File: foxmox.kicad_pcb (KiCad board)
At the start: 2 copper layers, 63.5 x 63.5 mm, 17 parts, among them P1 2.5mm plug, Q1 2N2222A, U1 PIC16F84, Y1 3.579MHz

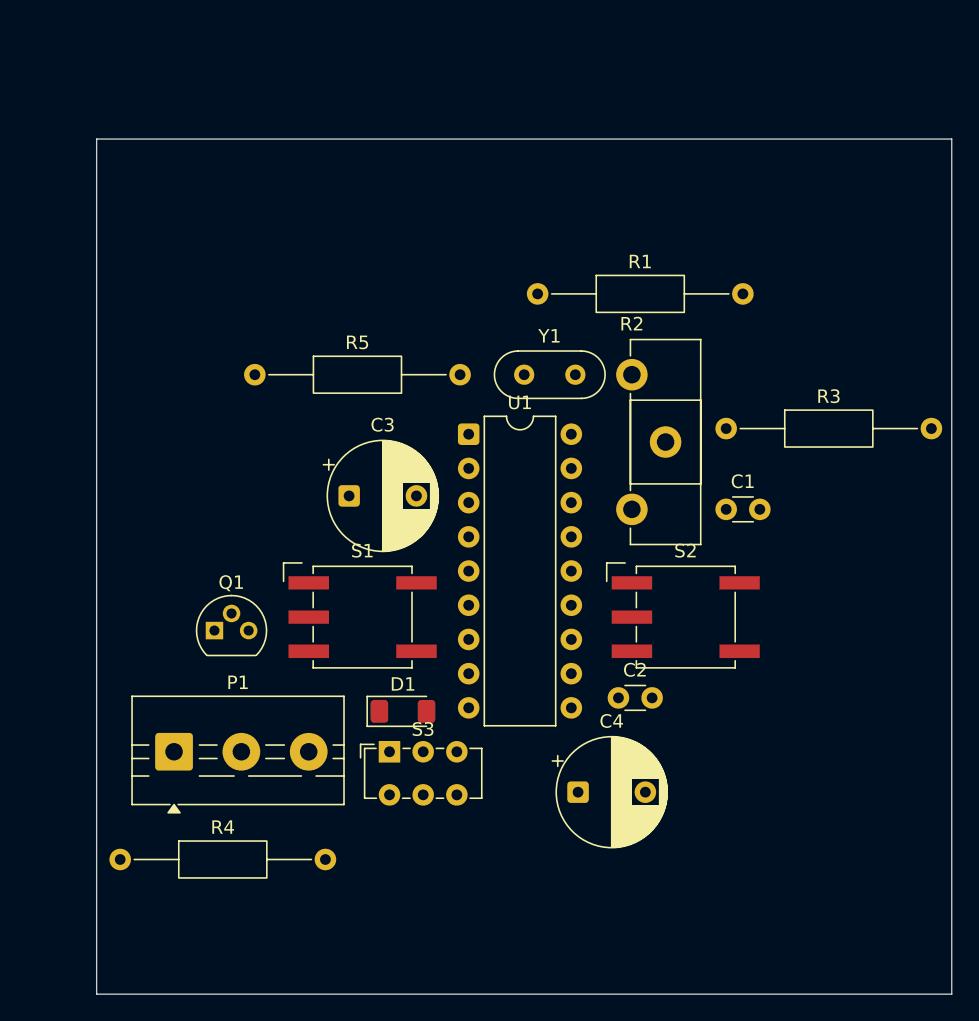
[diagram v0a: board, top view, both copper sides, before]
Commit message: Slightly better PCB
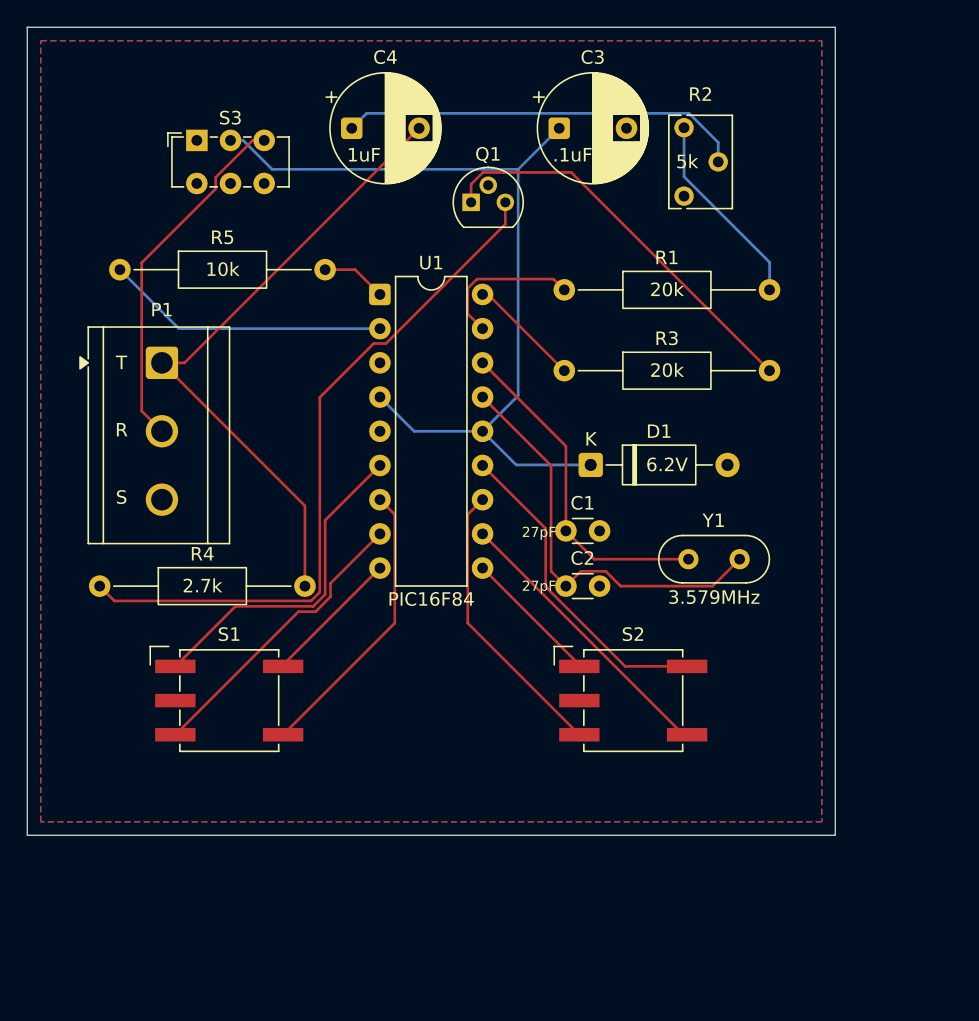
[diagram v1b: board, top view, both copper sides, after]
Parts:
- D1: footprint Diode_SMD:D_MiniMELF -> Diode_THT:D_A-405_P10.16mm_Horizontal
- P1: footprint TerminalBlock:TerminalBlock_MaiXu_MX126-5.0-03P_1x03_P5.00mm -> TerminalBlock_CUI:TerminalBlock_CUI_TB007-508-03_1x03_P5.08mm_Horizontal
- R2: footprint Potentiometer_THT:Potentiometer_Piher_PT-15-H01_Horizontal -> Potentiometer_THT:Potentiometer_Bourns_3266W_Vertical
- moved C4 52.1 mm to (134.1, 67.5)
- moved S3 47.6 mm to (122.6, 68.4)
- moved Q1 37.1 mm to (143.0, 73.0)
- moved C3 31.4 mm to (149.5, 67.5)
- moved P1 28.9 mm to (120.0, 84.9), turned to -90 degrees
- moved D1 23.0 mm to (151.8, 92.5)
- moved R4 20.4 mm to (115.4, 101.5)
- moved R2 18.7 mm to (158.8, 67.5), turned to 90 degrees
- moved Y1 18.3 mm to (159.1, 99.5)
- moved R3 12.8 mm to (149.9, 85.5)
- moved R5 12.7 mm to (116.9, 78.0)
- moved U1 12.3 mm to (136.2, 79.8)
- moved C1 12.0 mm to (150.0, 97.4)
- moved S1 11.7 mm to (125.0, 110.0)
- moved C2 9.17 mm to (150.0, 101.5)
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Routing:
- net Net-(D1-K): track 0.00 -> 64.8 mm, vias 0 -> 1
- net Net-(Q1-PadC): track 0.00 -> 52.3 mm
- net Net-(C4-Pad2): track 0.00 -> 47.3 mm
- net Net-(U1-OSC1/CLKIN): track 0.00 -> 31.2 mm
- net Net-(C4-Pad1): track 0.00 -> 30.0 mm
- net Net-(Q1-PadB): track 0.00 -> 30.0 mm
- net Net-(S3-C): track 0.00 -> 26.5 mm
- net Net-(U1-OSC2/CLKOUT): track 0.00 -> 25.0 mm
- net Net-(U1-INT/RB0): track 0.00 -> 24.6 mm
- net Net-(U1-RB7): track 0.00 -> 23.9 mm
- net Net-(U1-RB2): track 0.00 -> 22.0 mm
- net Net-(U1-RB5): track 0.00 -> 21.4 mm
- net Net-(U1-RB6): track 0.00 -> 21.3 mm
- net Net-(U1-RB1): track 0.00 -> 21.3 mm
- net Net-(U1-RA3): track 0.00 -> 21.1 mm
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- added copper zone on B.Cu, net GNDREF
- added copper zone on F.Cu, net GNDREF
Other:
- board size 63.5 x 63.5 mm -> 60 x 60 mm
